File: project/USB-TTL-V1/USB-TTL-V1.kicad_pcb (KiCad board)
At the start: 4 copper layers, 25.2 x 11.3 mm, 18 parts, among them J1 TTL-connect-pin4, J2 usbc, U1 CH340C, U2 SPX3819M5-L-3-3

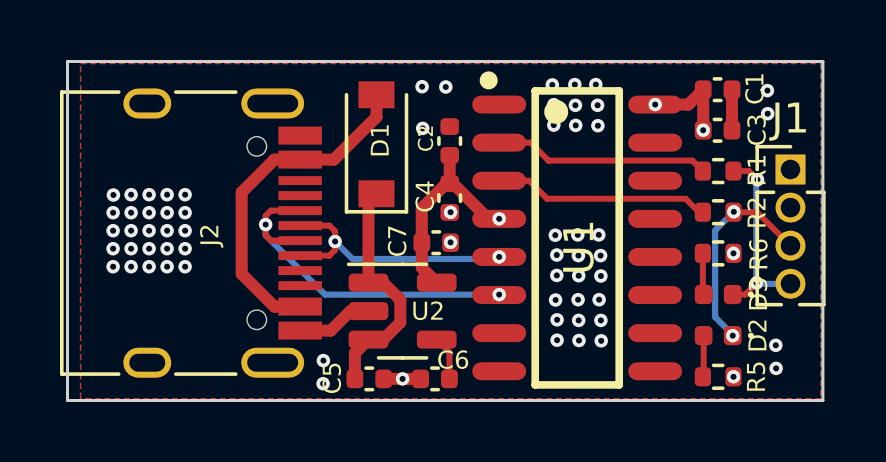
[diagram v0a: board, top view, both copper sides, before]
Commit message: fix: update screen  usb-ttl
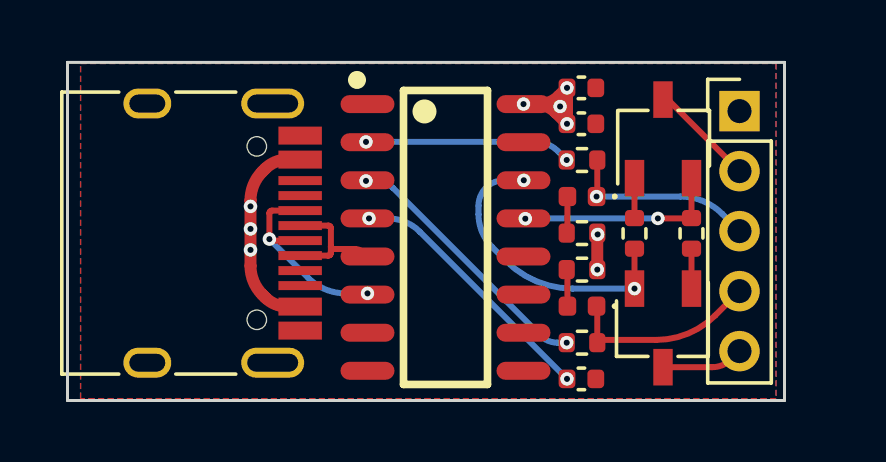
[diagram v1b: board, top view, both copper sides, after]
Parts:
- removed C4, C7: 10uf, Capacitor_SMD:C_0402_1005Metric
- removed C5: 1uf, Capacitor_SMD:C_0402_1005Metric
- removed C6: 470pf, Capacitor_SMD:C_0402_1005Metric
- removed D1: B120-E3, Diode_SMD:D_SOD-123
- removed U2: SPX3819M5-L-3-3, Package_TO_SOT_SMD:SOT-23-5
- added Q1: S8050, Package_TO_SOT_SMD:TSOT-23, F.Cu at (122.7, 90.5)
- added Q2: S8050, Package_TO_SOT_SMD:TSOT-23, F.Cu at (122.7, 84.2)
- added R3: 12K, Resistor_SMD:R_0402_1005Metric, F.Cu at (123.6, 87.3)
- added R4: 12K, Resistor_SMD:R_0402_1005Metric, F.Cu at (121.7, 87.3)
- J1: footprint Connector_PinHeader_1.27mm:PinHeader_1x04_P1.27mm_Vertical -> Connector_PinHeader_2.00mm:PinHeader_1x05_P2.00mm_Vertical
- R5, R6: value 1k -> 4.7k
- moved C3 9.45 mm to (119.9, 92.2)
- moved R2 6.29 mm to (120.0, 90.9)
- moved R5 5.78 mm to (120.0, 88.5)
- moved D3 5.59 mm to (120.0, 86.1)
- moved D2 4.65 mm to (120.0, 89.7)
- moved R6 4.59 mm to (120.0, 87.3)
- moved R1 4.55 mm to (120.0, 84.9)
- moved C1 4.54 mm to (119.9, 82.4)
- moved C2 4.43 mm to (119.9, 83.6), turned to 0 degrees
- moved U1 4.39 mm to (115.4, 87.4)
- moved J1 2.58 mm to (125.2, 83.2)
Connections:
- C1 pad 1: +3V3 -> +5V
- C2 pad 1: +3V3 -> +5V
- C3 pad 1: +3V3 -> Net-(C3-Pad1)
- J1 pad 2: GND -> /GPIO0
- J1 pad 3: /TXD -> /RXD
- J1 pad 4: /RXD -> /TXD
- J2 pad A4: Net-(D1-Pad2) -> +5V
- J2 pad A9: Net-(D1-Pad2) -> +5V
- J2 pad B4: Net-(D1-Pad2) -> +5V
- J2 pad B9: Net-(D1-Pad2) -> +5V
- R5 pad 1: +3V3 -> +5V
- R6 pad 1: +3V3 -> +5V
- U1 pad 13: unconnected-(U1-Pad13) -> Net-(Q2-Pad2)
- U1 pad 14: unconnected-(U1-Pad14) -> Net-(Q1-Pad2)
- U1 pad 16: +3V3 -> +5V
- U1 pad 4: +3V3 -> Net-(C3-Pad1)
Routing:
- net +3V3: track 26.1 -> 0.00 mm, vias 5 -> 0
- net +5V: track 0.00 -> 13.4 mm, vias 0 -> 9
- net Net-(D1-Pad2): track 11.4 -> 0.00 mm
- net Net-(Q1-Pad2): track 0.00 -> 9.98 mm, vias 0 -> 2
- net Net-(C3-Pad1): track 0.00 -> 8.79 mm, vias 0 -> 2
- net +5VD: track 7.92 -> 0.00 mm
- net Net-(Q2-Pad2): track 0.00 -> 6.94 mm, vias 0 -> 2
- net GND: track 5.32 -> 0.00 mm, vias 64 -> 0
- net Net-(J2-PadA7): track 12.1 -> 6.95 mm
- net Net-(J2-PadA6): track 8.84 -> 4.45 mm, vias 2 -> 0
- net /GPIO0: track 0.00 -> 3.53 mm
- net /EN: track 0.00 -> 2.73 mm
- net Net-(R2-Pad1): track 7.22 -> 8.90 mm, vias 0 -> 2
- net Net-(C6-Pad1): track 1.49 -> 0.00 mm
- net Net-(Q2-Pad1): track 0.00 -> 1.33 mm
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- added copper zone on In1.Cu, net +5V
- removed copper zone on In1.Cu, net GND
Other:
- board size 25.2 x 11.3 mm -> 23.9 x 11.3 mm
- board text added: "EN"
